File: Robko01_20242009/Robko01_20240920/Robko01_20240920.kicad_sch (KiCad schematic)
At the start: 78 parts, among them J1 Conn_01x04_Pin, J10 Motors, J11 Motors, J12 Conn_01x04_Pin, J13 Conn_01x02_Pin, J14 Conn_01x04_Pin, J15 Conn_01x02_Pin, J16 Conn_01x04_Pin, J17 Conn_01x02_Male, J18 Conn_01x02_Male, J19 Conn_01x02_Male, J2 Conn_01x02_Pin, J20 Conn_01x02_Male, J21 Conn_01x19_Pin, J22 Conn_01x19_Pin, J23 Conn_02x05_Odd_Even, J28 Conn_01x02_Male, J29 Conn_01x07_Pin, J3 Conn_01x02_Pin, J30 Conn_01x02_Male, J31 Conn_02x05_Odd_Even, J4 Conn_01x04_Pin, J5 Conn_01x02_Pin, J6 Conn_01x04_Pin, J7 Conn_01x02_Male, J8 Conn_01x02_Pin, J9 Motors, K2 G5V-2, SW1 SW_DIP_x04, SW2 SW_DIP_x04, SW3 SW_DIP_x04, SW4 SW_DIP_x04, SW5 SW_DIP_x04, SW7 SW_DIP_x04, U1 LM7805_TO220, U2 PC817

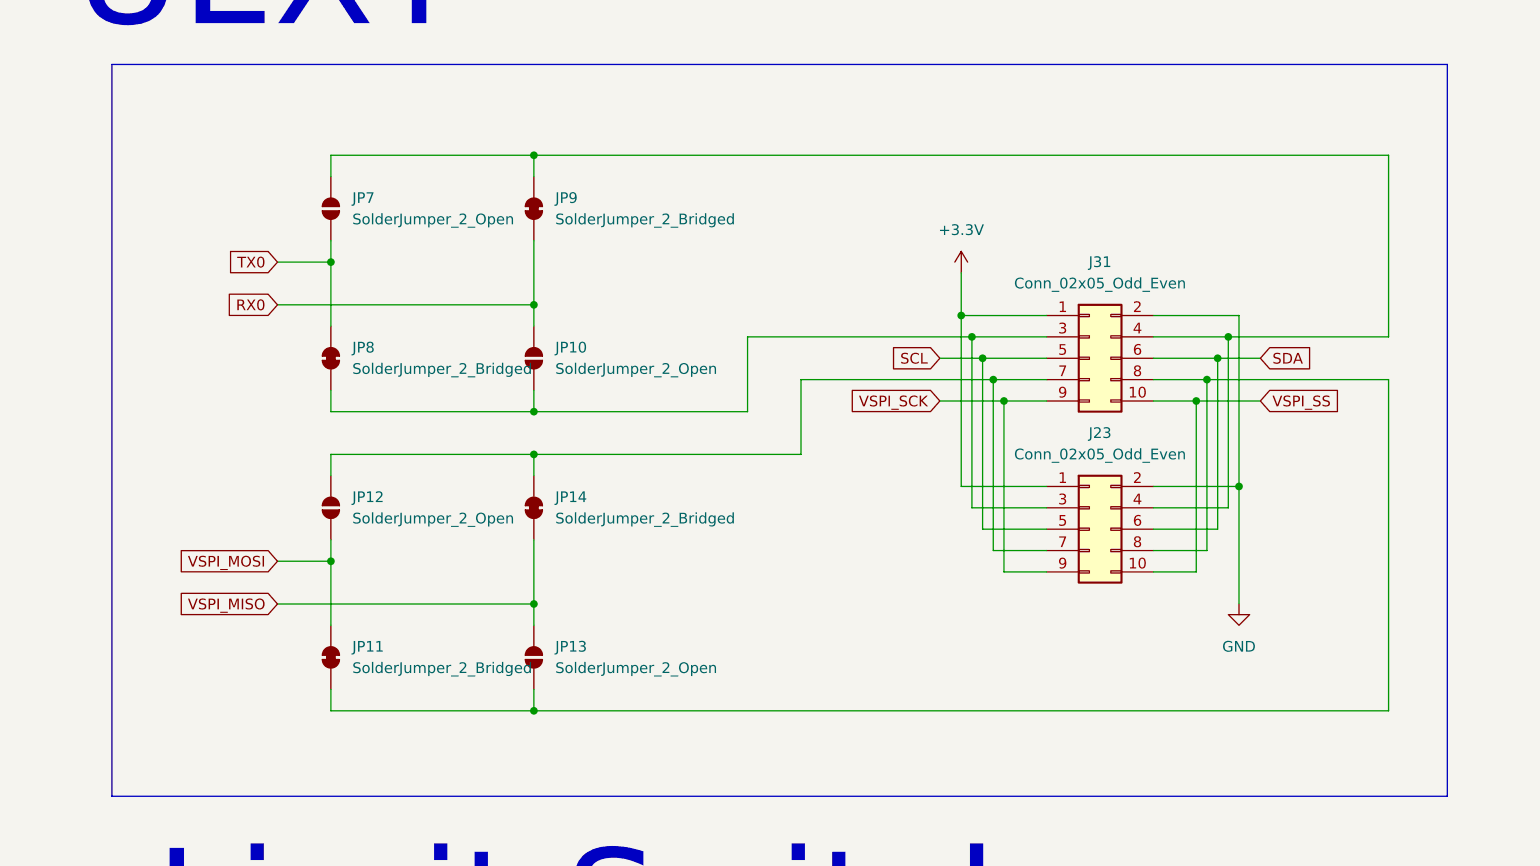
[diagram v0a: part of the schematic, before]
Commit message: Change jumpers for UEXT
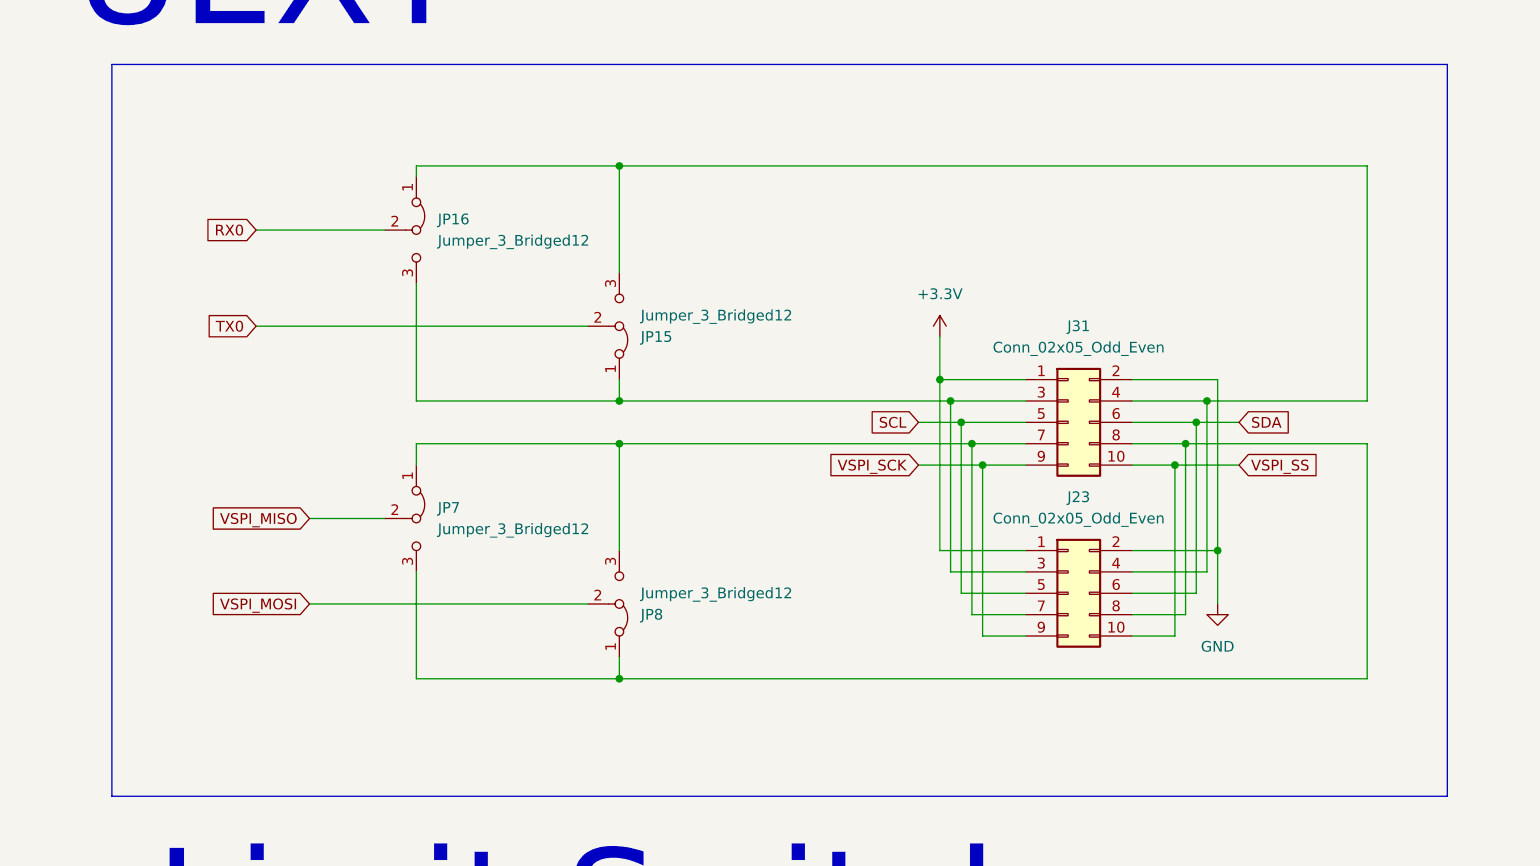
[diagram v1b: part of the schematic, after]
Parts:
- removed JP10, JP12, JP13, JP7: SolderJumper_2_Open, Jumper:SolderJumper-2_P1.3mm_Open_RoundedPad1.0x1.5mm, symbol Jumper:SolderJumper_2_Open
- removed JP11, JP14, JP8, JP9: SolderJumper_2_Bridged, Jumper:SolderJumper-2_P1.3mm_Bridged2Bar_RoundedPad1.0x1.5mm, symbol Jumper:SolderJumper_2_Bridged
- added JP15, JP16, JP7, JP8: Jumper_3_Bridged12, Jumper:SolderJumper-3_P1.3mm_Bridged2Bar12_Pad1.0x1.5mm, symbol Jumper:Jumper_3_Bridged12
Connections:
- net RX0: now also JP16.2 (C)
- net TX0: now also JP15.2 (C)
- net VSPI_MISO: now also JP7.2 (C)
- net VSPI_MOSI: now also JP8.2 (C)
- net at J23.3 (Pin_3), J31.3 (Pin_3): now also JP15.1 (A), JP16.3 (B)
- net at J23.4 (Pin_4), J31.4 (Pin_4): now also JP15.3 (B), JP16.1 (A)
- net at J23.7 (Pin_7), J31.7 (Pin_7): now also JP7.1 (A), JP8.3 (B)
- net at J23.8 (Pin_8), J31.8 (Pin_8): now also JP7.3 (B), JP8.1 (A)
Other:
- moved on the sheet: J23, J31
